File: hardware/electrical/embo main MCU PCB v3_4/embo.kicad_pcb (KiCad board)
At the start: 4 copper layers, 96.4 x 76.1 mm, 129 parts, among them IC1 OPA2354, IC2 OPA2354, J1 Conn_Coaxial, J13 USB_C_Receptacle_USB2.0_16P, J14 24 V PSU input, J15_1 Conn_01x04, J15_2 Conn_01x04, J16 3.3V out, J2 Conn_Coaxial, J3 Conn_01x03, J4 Conn_01x04, J5 Conn_01x04, J6 motor 1, J7 motor 2, J8 5V out, J9 Conn_02x10_Odd_Even, M3 MountingHole_3.2mm_M3, Q1 AO4407A, U1 ESP32-S3-WROOM-1, U2 LM2596S-5, U3 AMS1117-3.3

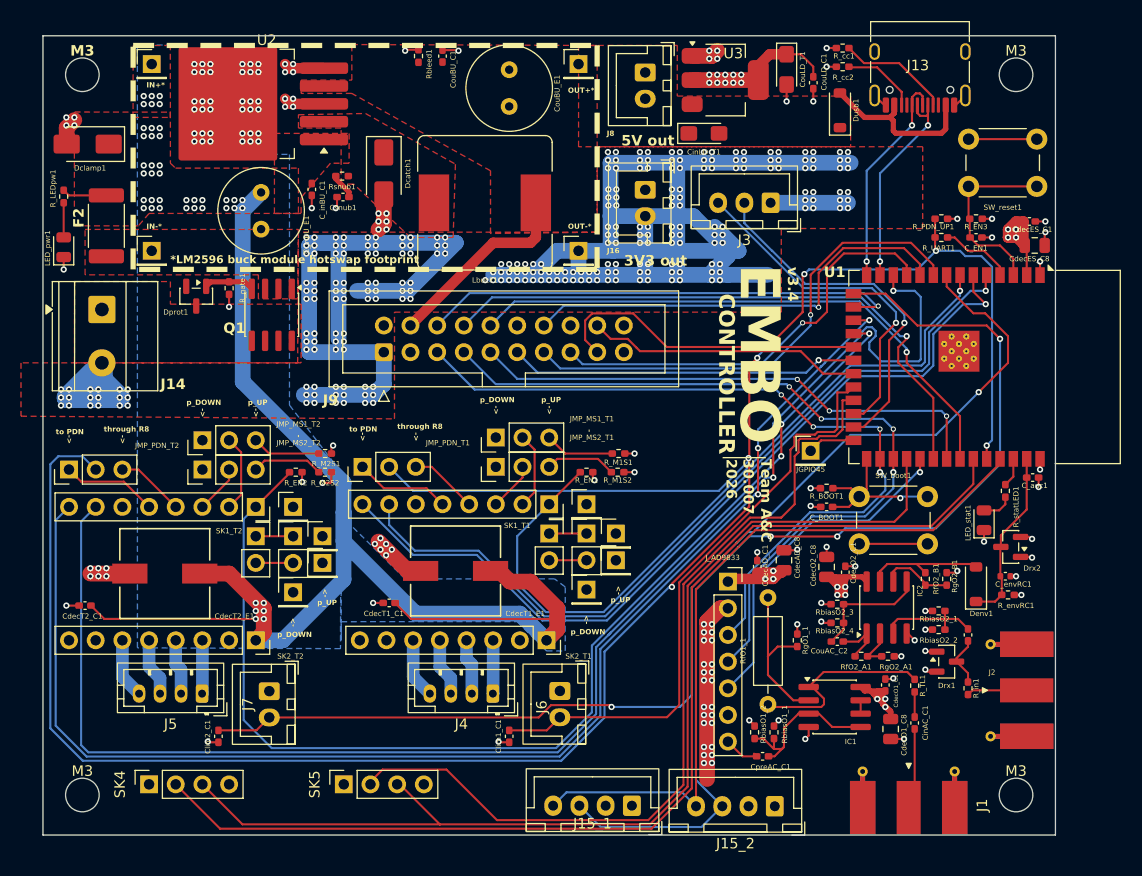
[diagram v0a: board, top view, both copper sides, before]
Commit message: v3.4 PCb final changes
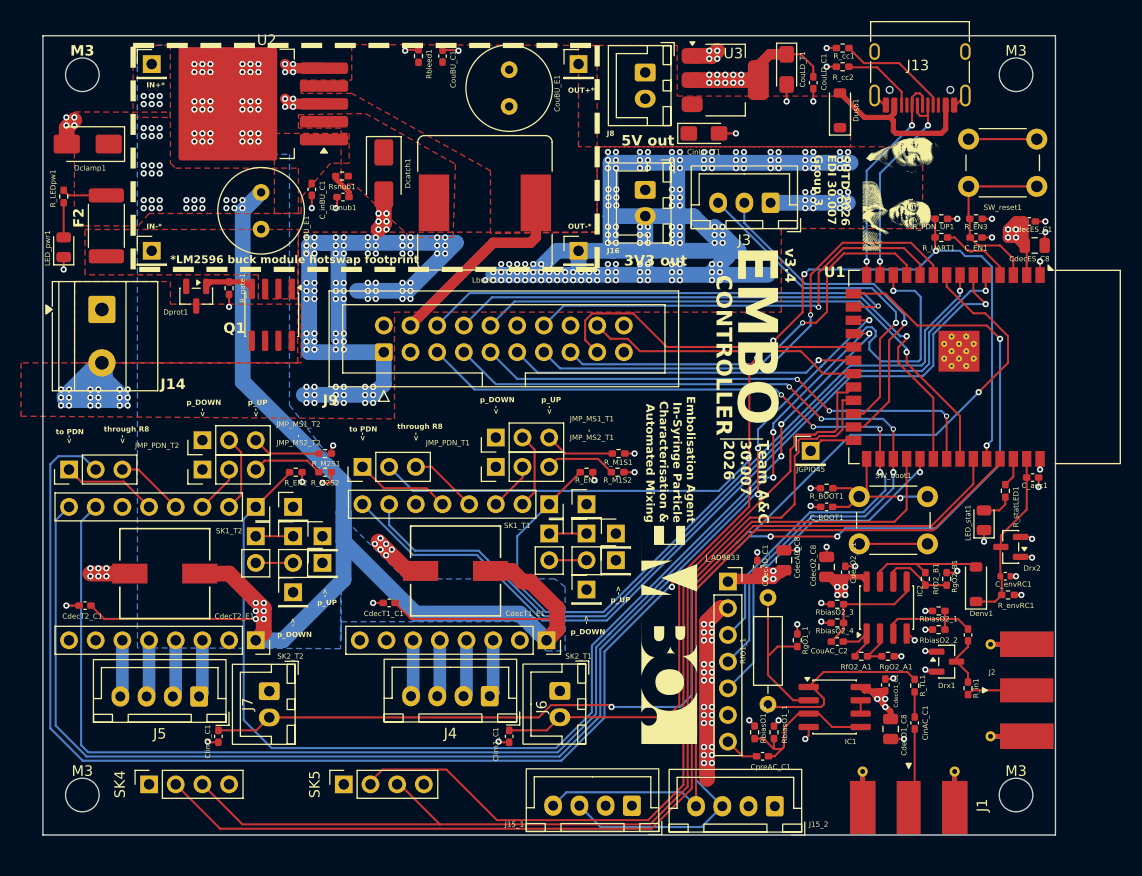
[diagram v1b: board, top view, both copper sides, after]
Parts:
- added G***: LOGO, EMBO_Custom_Footprints:EMBO LOGO, F.Cu at (148.1, 116.7)
- added G***: LOGO, EMBO_Custom_Footprints:PROFS2, F.Cu at (170.4, 74.4)
- added G***: LOGO, EMBO_Custom_Footprints:EMBO7, B.Cu at (141.3, 98.3)
- J4, J5: footprint Connector_JST:JST_PH_B4B-PH-K_1x04_P2.00mm_Vertical -> Connector_JST:JST_XH_B4B-XH-A_1x04_P2.50mm_Vertical
- moved J5 0.39 mm to (103.3, 123.2)
- moved J4 0.38 mm to (131.0, 123.2)
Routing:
- net GND: track 307.5 -> 309.1 mm, vias 391 -> 392
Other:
- board text added: "Embolisation Agent In-Syringe Particle Characterisation & Automated Mixing"
- board text added: "SUTD 2026 EDI 30.007 Group 3"
